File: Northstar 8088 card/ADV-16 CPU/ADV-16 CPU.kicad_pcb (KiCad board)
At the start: 2 copper layers, 228.1 x 165.3 mm, 113 parts, among them J1 Power In, J2 Conn_01x16_Socket, J3 Conn_01x18_Socket, P1 northstar card edge, Q1 2N3904, U1 74LS175, U10 74LS155, U11 74LS373, U12 8088-2, U13 74LS00, U14 74LS04, U15 74LS393, U16 74S08, U17 8284, U18 74LS258, U19 74LS174, U2 74S112, U20 74LS03, U21 74LS153, U22 74LS74, U23 74S00, U24 74LS393, U25 74LS244, U26 74LS258, U27 6309-1, U28 74LS373, U29 74LS245, U3 85ns_Delay, U30 74LS244, U31 74LS10, U32 4164, U33 4164, U34 4164, U35 4164, U36 4164, U37 4164, U38 4164, U39 4164, U4 74S04, U40 4164, U41 74LS280, U42 74LS374, U43 74LS373, U44 74LS138, U5 74LS32, U6 74LS74, U7 74LS20, U8 74LS74, U9 74LS00, Y1 24MHz

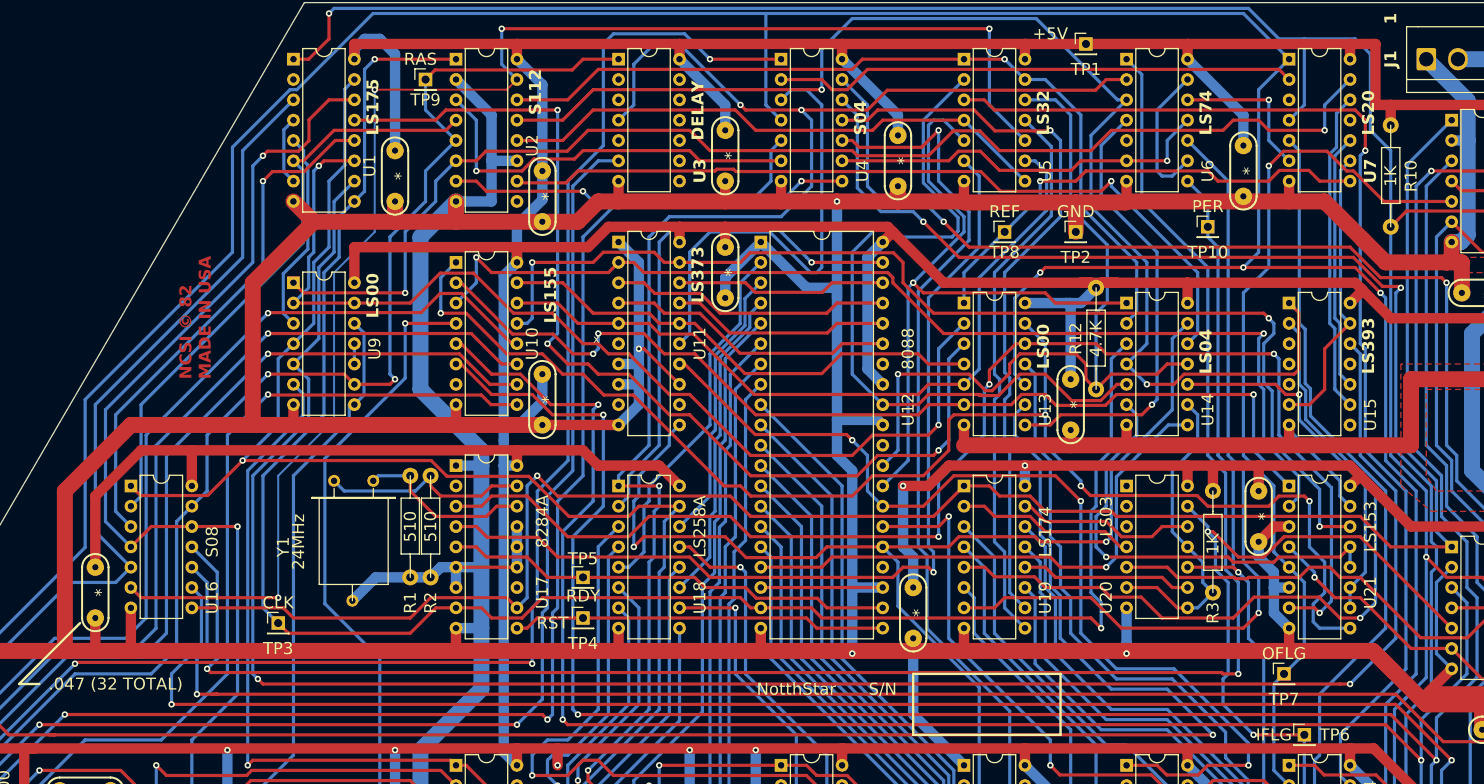
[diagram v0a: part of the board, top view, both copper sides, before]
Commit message: tweaks for production
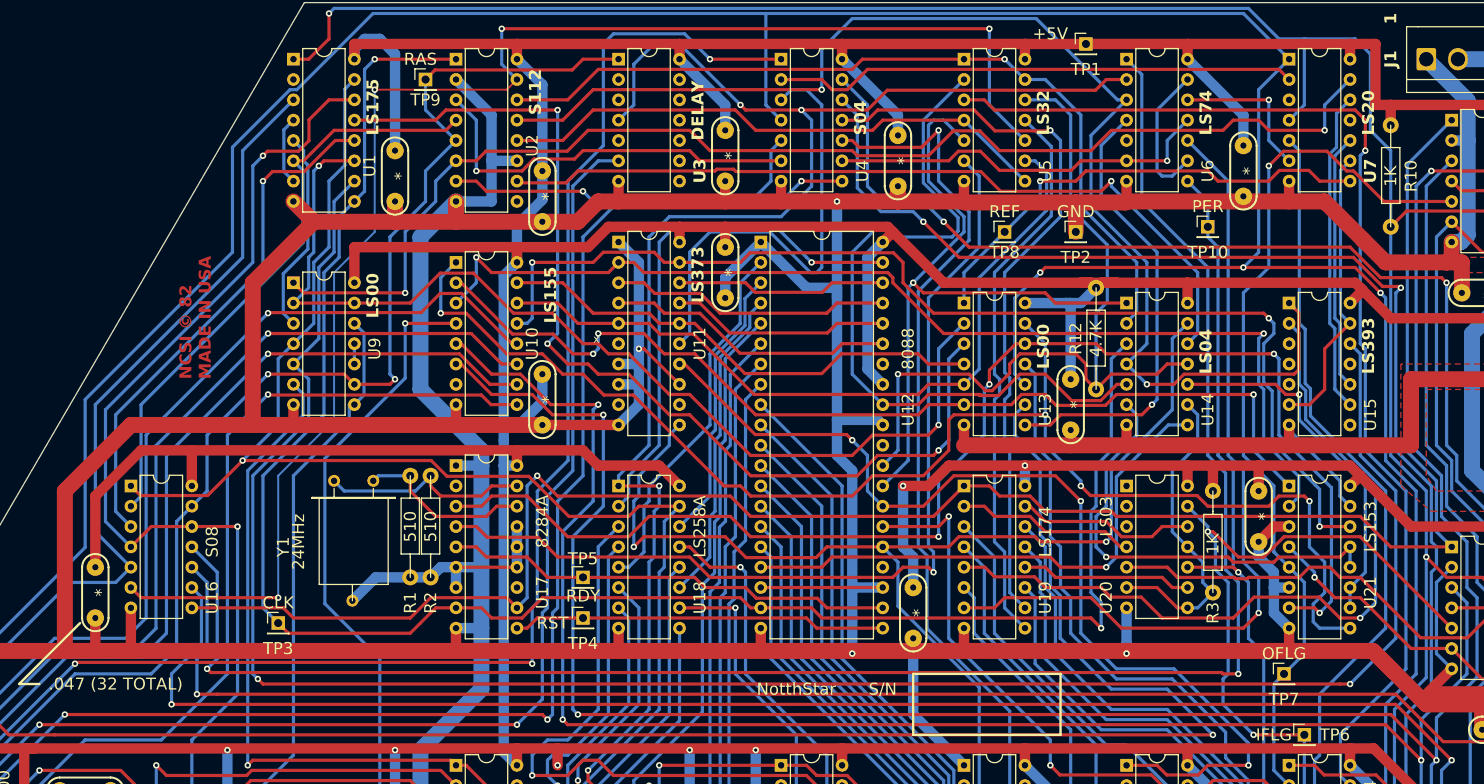
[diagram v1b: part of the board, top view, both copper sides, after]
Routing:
- net Net-(U16-Pad10): track 208.9 -> 208.3 mm
- net Net-(U1-~{Q0}): track 313.2 -> 312.5 mm
- net PUP2: track 339.4 -> 338.8 mm
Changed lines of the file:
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@@
     (fp_line (start 10.27 4.05) (end 10.27 -3.95)
       (stroke (width 0.1) (type solid)) (layer "F.Fab"))
-    (pad "1" thru_hole roundrect (at 0 0) (size 2.46 2.8) (drill 1.8) (layers "*.Cu" "*.Mask") (roundrect_rratio 0.101626)
+    (pad "1" thru_hole roundrect (at 0 0) (size 2.46 2.8) (drill 1.8) (layers "*.Cu" "*.Mask") (roundrect_rratio 0.1016260163)
       (net 2 "GND") (pinfunction "Pin_1") (pintype "passive"))
     (pad "2" thru_hole oval (at 3.96 0) (size 2.46 2.8) (drill 1.8) (layers "*.Cu" "*.Mask")
@@
   (via (at 104.14 20.955) (size 0.8) (drill 0.4) (layers "F.Cu" "B.Cu") (net 41))
   (via (at 234.95 148.59) (size 0.8) (drill 0.4) (layers "F.Cu" "B.Cu") (net 41))
-  (segment (start 238.76 106.515) (end 238.36 106.915) (width 0.4) (layer "B.Cu") (net 41))
   (segment (start 252.095 97.79) (end 254 95.885) (width 0.4) (layer "B.Cu") (net 41))
   (segment (start 254 95.885) (end 254 94.615) (width 0.4) (layer "B.Cu") (net 41))
@@
   (segment (start 217.805 90.805) (end 219.075 92.075) (width 0.4) (layer "B.Cu") (net 59))
   (segment (start 58.42 105.41) (end 64.135 111.125) (width 0.4) (layer "F.Cu") (net 61))
-  (segment (start 69.215 111.125) (end 69.85 111.125) (width 0.4) (layer "F.Cu") (net 61))
   (segment (start 69.85 111.125) (end 214.63 111.125) (width 0.4) (layer "F.Cu") (net 61))
   (segment (start 64.135 111.125) (end 69.85 111.125) (width 0.4) (layer "F.Cu") (net 61))
@@
   (segment (start 243.425 111.98) (end 251.24 111.98) (width 0.4) (layer "F.Cu") (net 162))
   (segment (start 90.17 106.045) (end 87.63 106.045) (width 0.4) (layer "F.Cu") (net 162))
-  (segment (start 89.535 106.045) (end 90.17 106.045) (width 0.4) (layer "F.Cu") (net 162))
   (segment (start 90.17 106.045) (end 237.49 106.045) (width 0.4) (layer "F.Cu") (net 162))
   (segment (start 251.24 111.98) (end 252.095 111.125) (width 0.4) (layer "F.Cu") (net 162))
